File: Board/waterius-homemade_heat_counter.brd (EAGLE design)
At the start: 50.5 x 61.6 mm, 38 parts, among them IC1 TINY13-20SU, Q1 MMBTA92, Q2 MMBTA92, U1 RS-485-MODULE

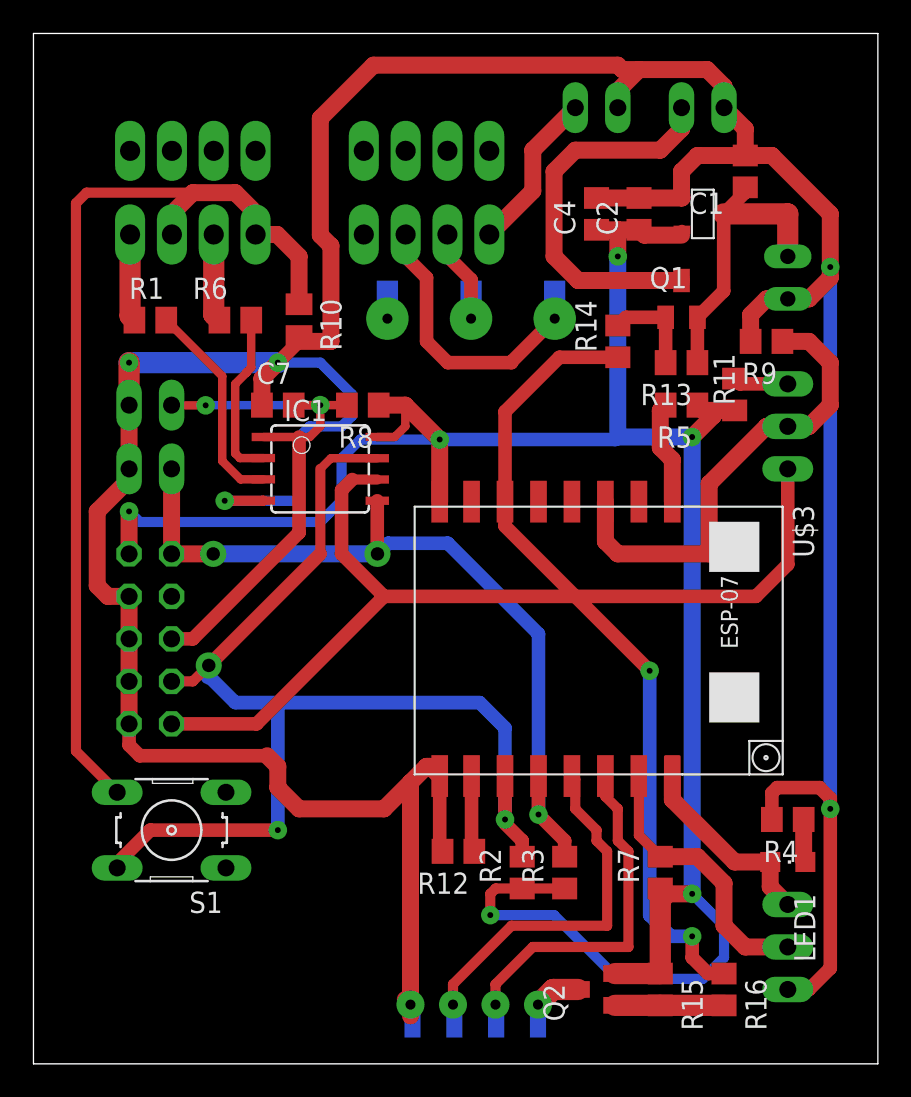
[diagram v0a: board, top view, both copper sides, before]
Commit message: rewire1
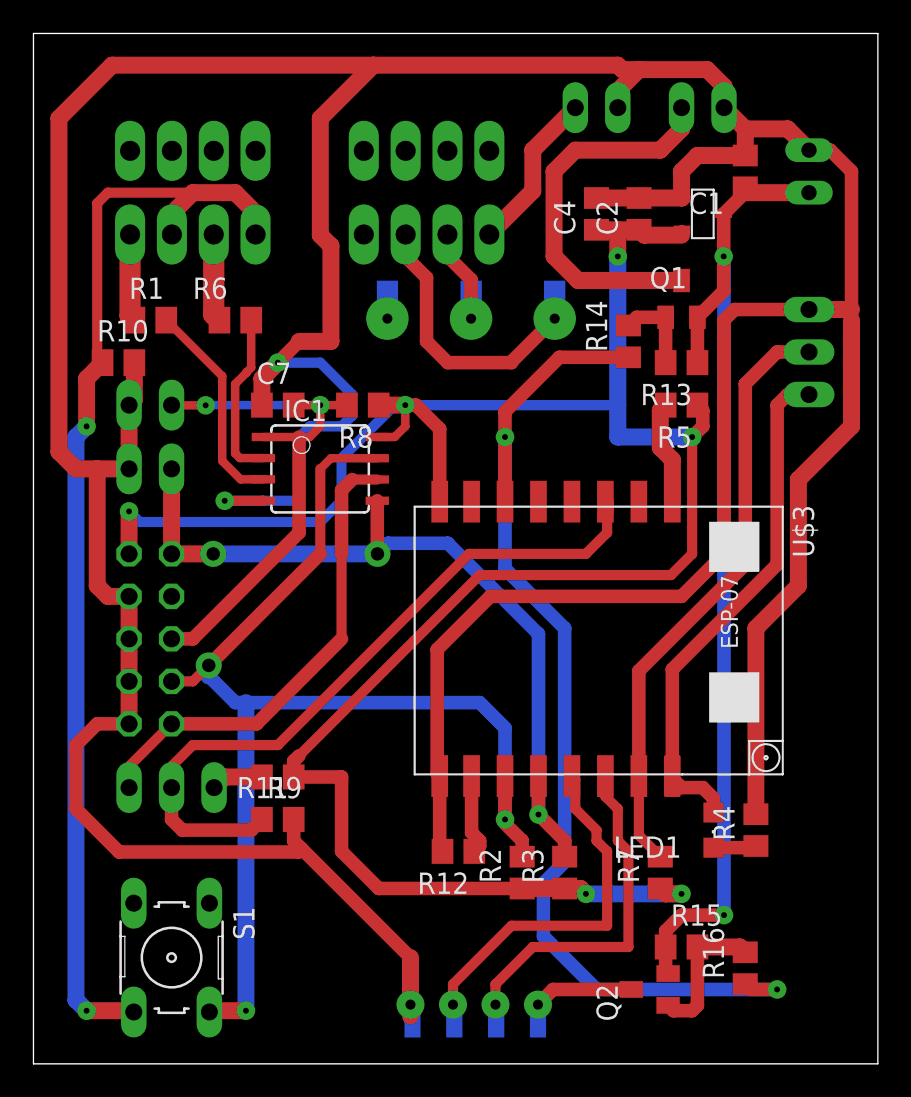
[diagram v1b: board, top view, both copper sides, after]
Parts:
- moved JP4 42.7 mm to (11.4, 33.0), turned to 0 degrees
- moved R9 40.9 mm to (17.8, 31.1), turned to 0 degrees
- moved R11 35.6 mm to (17.8, 33.7), turned to 180 degrees
- moved JP5 35.6 mm to (49.5, 59.1), turned to 90 degrees
- moved R10 11.1 mm to (8.26, 58.4), turned to 0 degrees
- moved S1 7.62 mm to (11.4, 22.9), turned to 270 degrees
- moved JP1 6.48 mm to (49.5, 69.8), turned to 180 degrees
- moved LED1 4.84 mm to (43.8, 30.5), turned to 180 degrees
- moved Q2 3.18 mm to (40.0, 21.0)
- moved R15 2.84 mm to (41.9, 23.5), turned to 0 degrees
- moved R4 2.01 mm to (46.4, 30.5), turned to 90 degrees
- moved R16 1.80 mm to (45.7, 22.2), turned to 90 degrees
- moved R14 0.63 mm to (38.7, 59.7)
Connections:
- net +3V3: no longer Q2.2, R15.1
- net AA*3: now also Q2.2, R15.1
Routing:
- net GND: track 230.7 -> 292.8 mm, vias 5 -> 2
- net AA*3: track 18.0 -> 61.4 mm, vias 0 -> 2
- net WAKE_UP: track 56.3 -> 28.4 mm
- net N$5: track 16.7 -> 36.0 mm
- net N$1: track 11.8 -> 30.9 mm
- net EN_HC_VCC: track 48.4 -> 63.3 mm
- net N$7: track 28.2 -> 42.8 mm
- net GND1: track 58.1 -> 66.8 mm, vias 0 -> 2
- net VCC_RS485: track 4.23 -> 6.95 mm
- net +3V3: track 137.3 -> 139.8 mm
- net SCK: track 69.5 -> 71.8 mm
- net N$13: track 6.52 -> 8.51 mm
- net RS485_B: track 7.69 -> 6.61 mm
- net N$10: track 5.77 -> 5.14 mm
